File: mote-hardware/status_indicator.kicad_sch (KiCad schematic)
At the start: 8 parts

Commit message: Switch to blue LEDs
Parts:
- D1, D2: LCSC C2290 -> C2288
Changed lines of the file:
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@@
 			)
 		)
-		(property "LCSC" "C2290"
+		(property "LCSC" "C2288"
 			(at 204.47 97.79 90)
 			(effects
@@
 			)
 		)
-		(property "LCSC" "C2290"
+		(property "LCSC" "C2288"
 			(at 215.9 97.79 90)
 			(effects

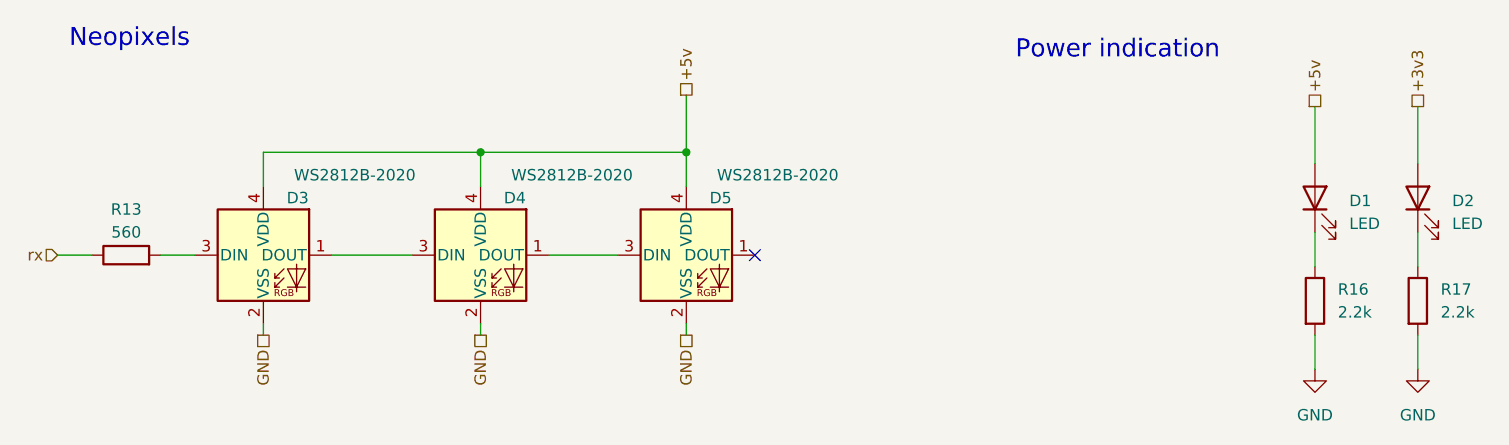
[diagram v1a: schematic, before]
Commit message: Add comments to schematic, respect ground pin on SWD and UART connectors
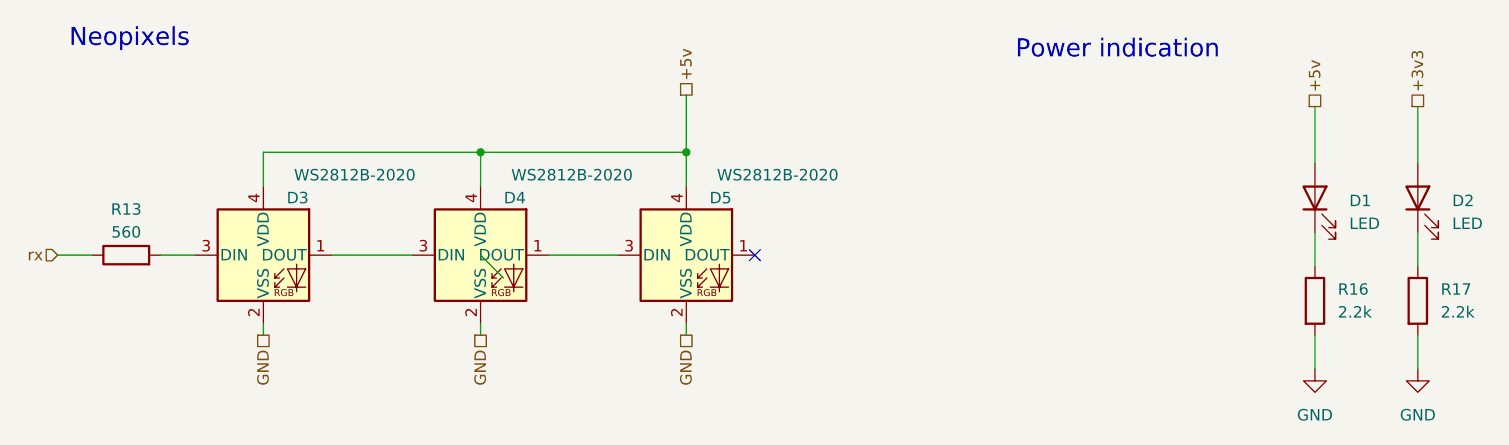
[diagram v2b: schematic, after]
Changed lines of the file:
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@@
 		(at 142.24 104.14)
+	)
+	(bus_entry
+		(at 111.76 104.14)
+		(size 2.54 2.54)
+		(stroke
+			(width 0)
+			(type default)
+		)
 	)
 	(wire

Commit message: Add position corrections
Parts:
- D1, D2, R13, R16, R17: JLCPCB_CORRECTION (none) -> 0; 0; 0
- D3, D4, D5: JLCPCB_CORRECTION (none) -> 0; 0; 90
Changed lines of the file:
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@@
 			)
 		)
-		(property "JLCPCB_CORRECTION" ""
+		(property "JLCPCB_CORRECTION" "0; 0; 0"
 			(at 72.39 104.14 90)
 			(effects
@@
 			)
 		)
-		(property "JLCPCB_CORRECTION" ""
+		(property "JLCPCB_CORRECTION" "0; 0; 0"
 			(at 204.47 97.79 90)
 			(effects
@@
 			)
 		)
-		(property "JLCPCB_CORRECTION" ""
+		(property "JLCPCB_CORRECTION" "0; 0; 90"
 			(at 134.62 104.14 0)
 			(effects
@@
 			)
 		)
-		(property "JLCPCB_CORRECTION" ""
+		(property "JLCPCB_CORRECTION" "0; 0; 90"
 			(at 87.63 104.14 0)
 			(effects
@@
 			)
 		)
-		(property "JLCPCB_CORRECTION" ""
+		(property "JLCPCB_CORRECTION" "0; 0; 90"
 			(at 111.76 104.14 0)
 			(effects
@@
 			)
 		)
-		(property "JLCPCB_CORRECTION" ""
+		(property "JLCPCB_CORRECTION" "0; 0; 0"
 			(at 215.9 109.22 0)
 			(effects
@@
 			)
 		)
-		(property "JLCPCB_CORRECTION" ""
+		(property "JLCPCB_CORRECTION" "0; 0; 0"
 			(at 204.47 109.22 0)
 			(effects
@@
 			)
 		)
-		(property "JLCPCB_CORRECTION" ""
+		(property "JLCPCB_CORRECTION" "0; 0; 0"
 			(at 215.9 97.79 90)
 			(effects
